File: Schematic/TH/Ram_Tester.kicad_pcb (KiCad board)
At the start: 2 copper layers, 63.3 x 57.2 mm, 42 parts, among them J1 Conn_01x02_Pin, J2 ICSP, Q1 2N7000, Q2 2N7000, SW1 SW_DIP_x03, SW2 SW_Push, U1 ATmega328-P, U2 RAM / ZIF, U3 ZIP Socket, Y1 Crystal

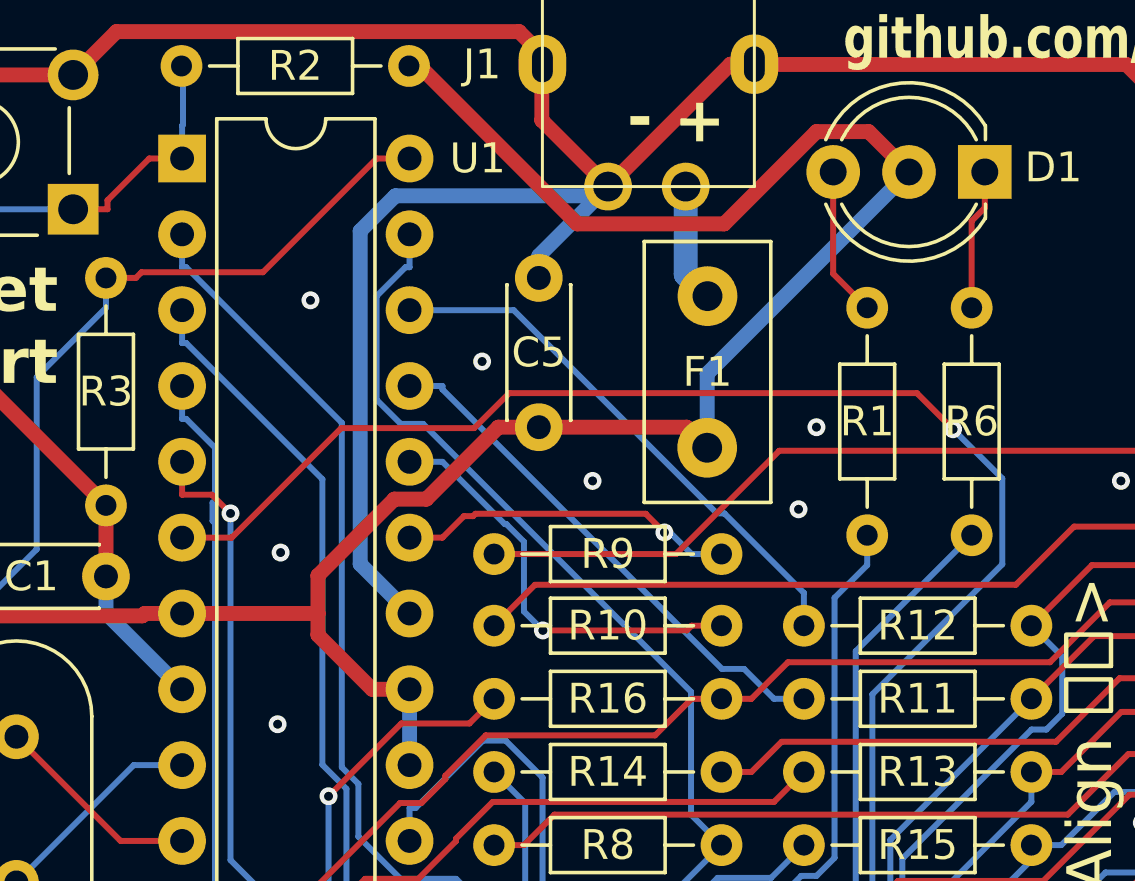
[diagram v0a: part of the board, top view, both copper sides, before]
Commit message: v1.1 - minor fix
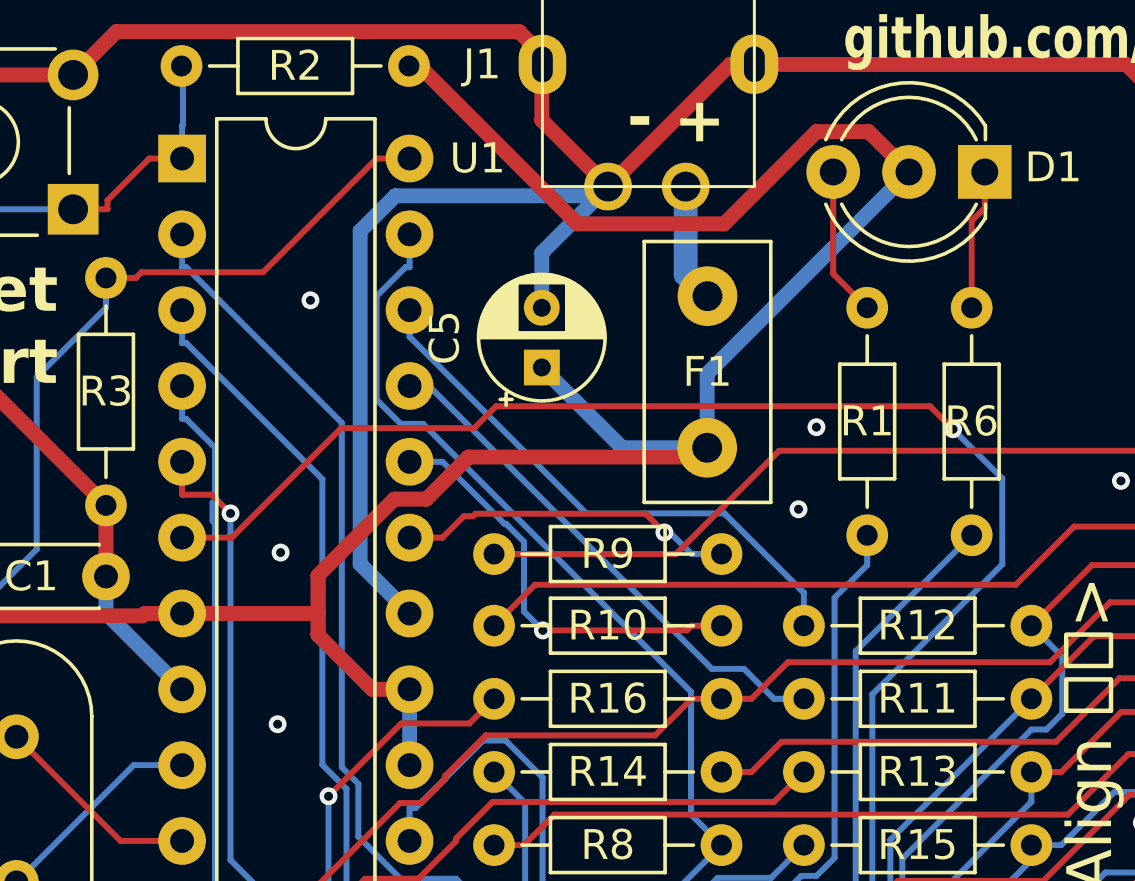
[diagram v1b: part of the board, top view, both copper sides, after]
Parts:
- C5: footprint Capacitor_THT:C_Disc_D4.3mm_W1.9mm_P5.00mm -> Capacitor_THT:CP_Radial_D4.0mm_P2.00mm
- moved C5 2.00 mm to (117.6, 77.0)
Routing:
- net /5V: track 124.3 -> 130.3 mm
- net /GND: track 198.9 -> 199.9 mm, vias 40 -> 38
- net Net-(U1-PC3): track 18.2 -> 18.8 mm
